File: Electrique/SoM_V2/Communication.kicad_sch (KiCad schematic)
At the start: 30 parts, among them U301 TCA9546APWR, U302 FT231XQ, U305 SN65HVD230

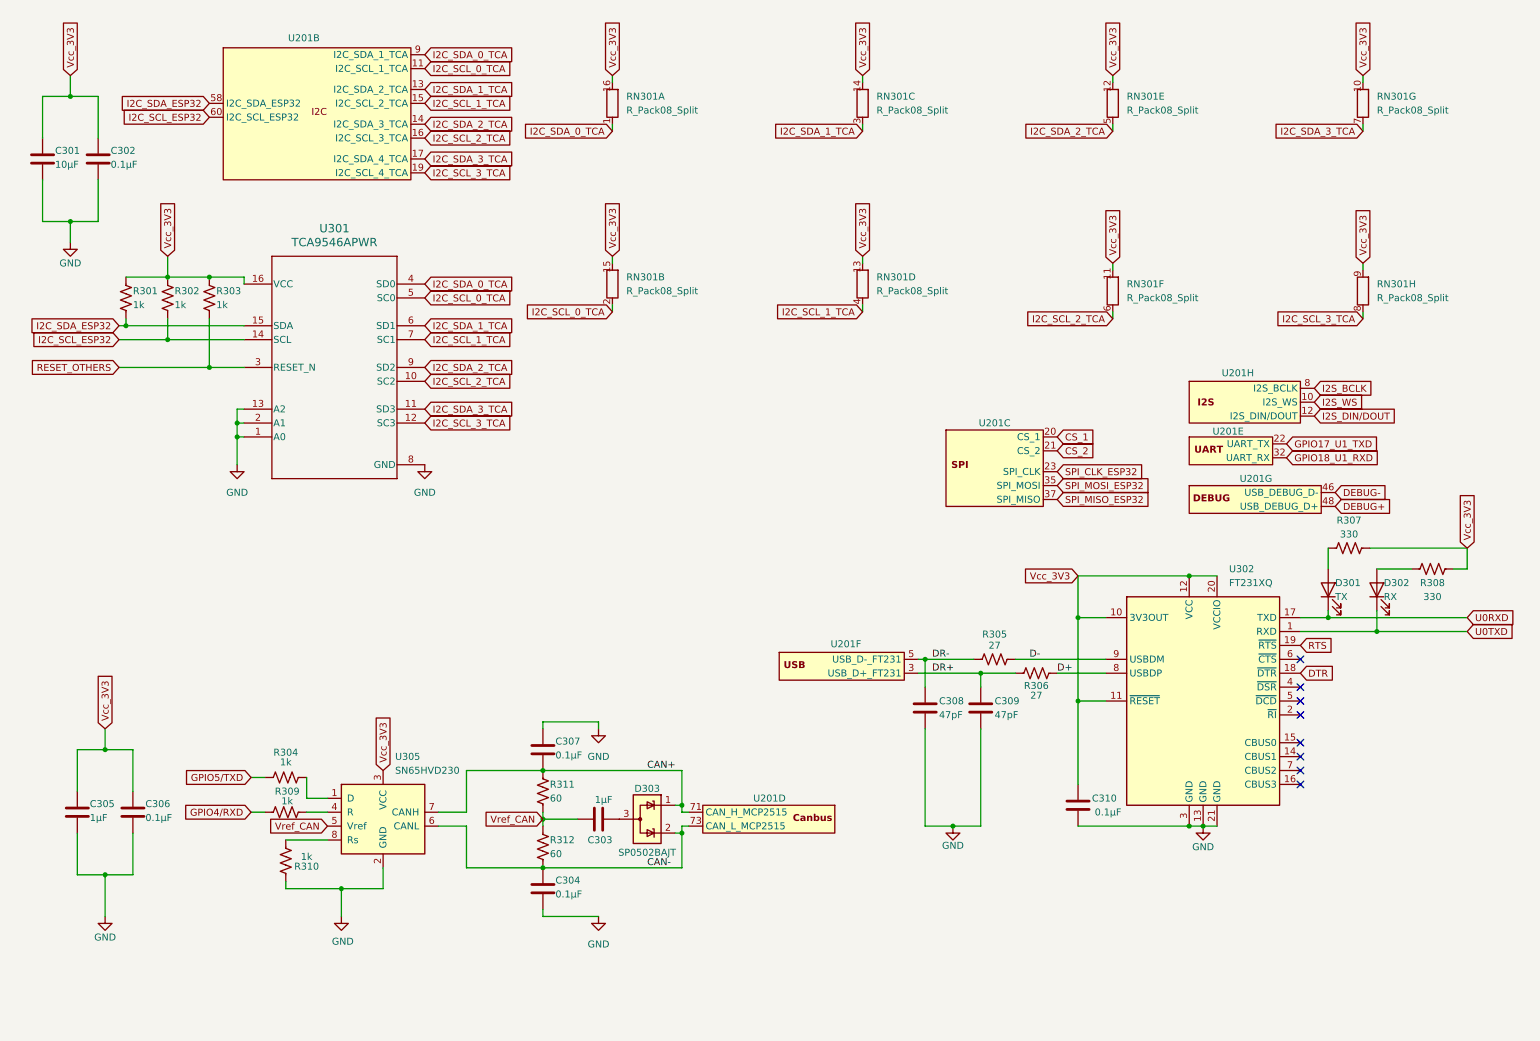
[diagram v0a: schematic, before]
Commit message: Clean up schema et PCB
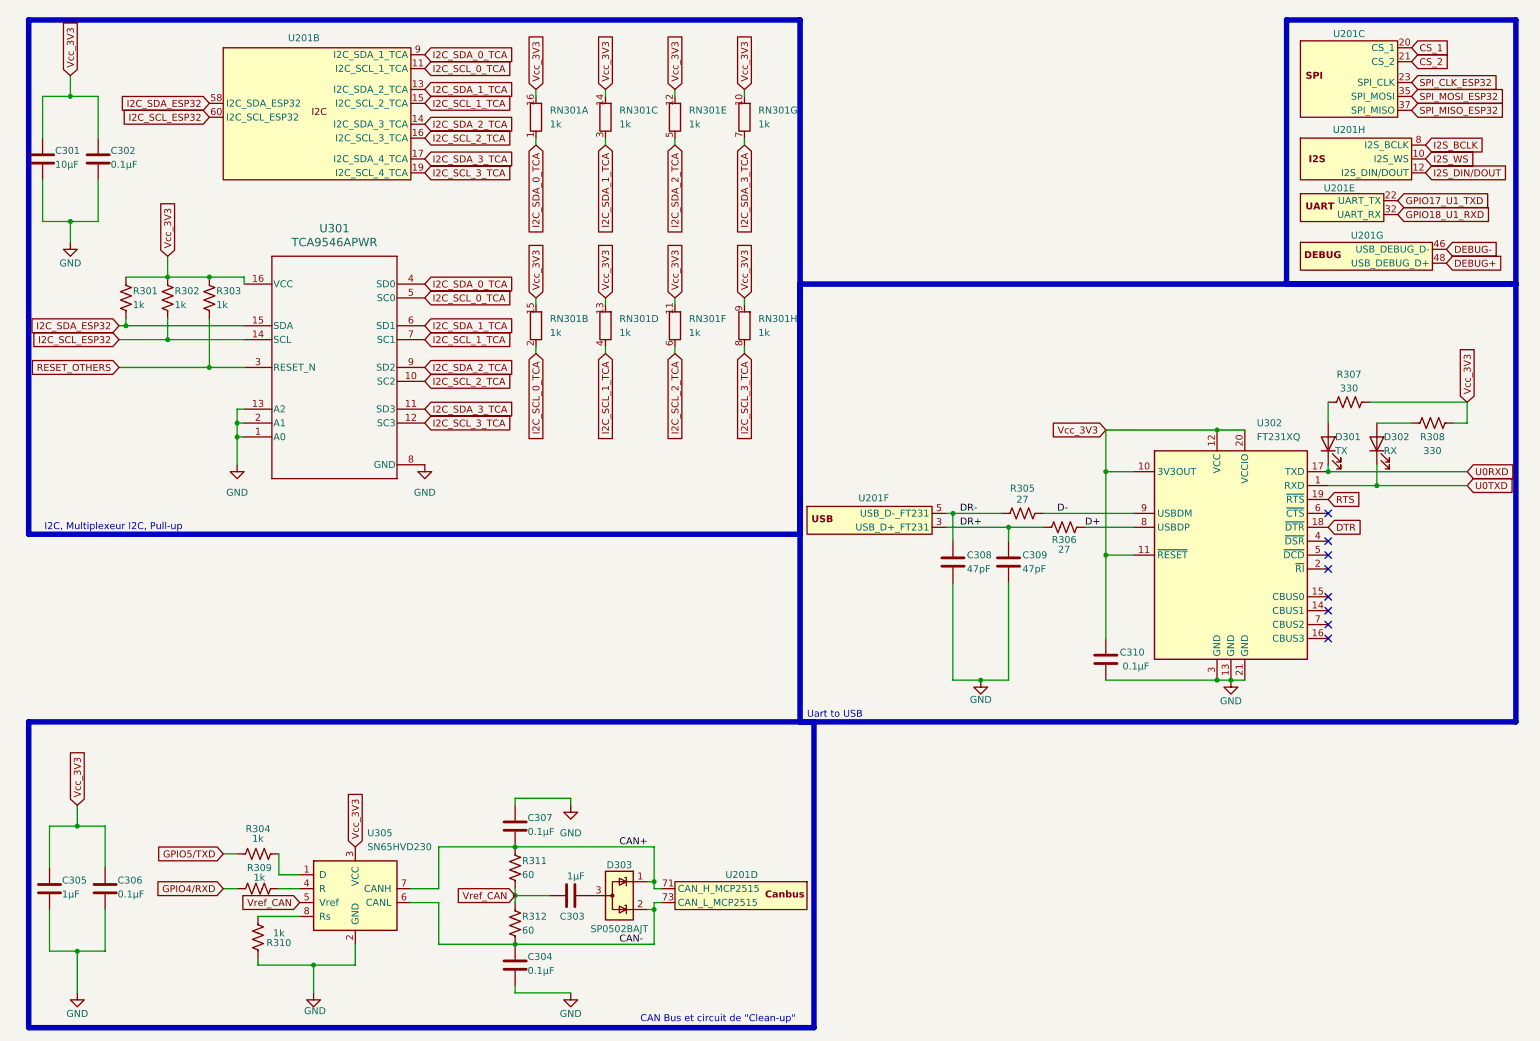
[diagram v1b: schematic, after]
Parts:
- RN301: value R_Pack08_Split -> 1k
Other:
- note added: "CAN Bus et circuit de "Clean-up""
- note added: "I2C, Multiplexeur I2C, Pull-up"
- note added: "Uart to USB"
- moved on the sheet: C303, C304, C305, C306, C307, C308, C309, C310, D301, D302, D303, R304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
